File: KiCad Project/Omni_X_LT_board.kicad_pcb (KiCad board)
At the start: 2 copper layers, 64.8 x 25.5 mm, 32 parts, among them J1 Conn_01x02_Female, J2 Conn_01x02_Female, U1 TLV9001IDCK, U2 TLV9001IDCK, U3 ADS1110

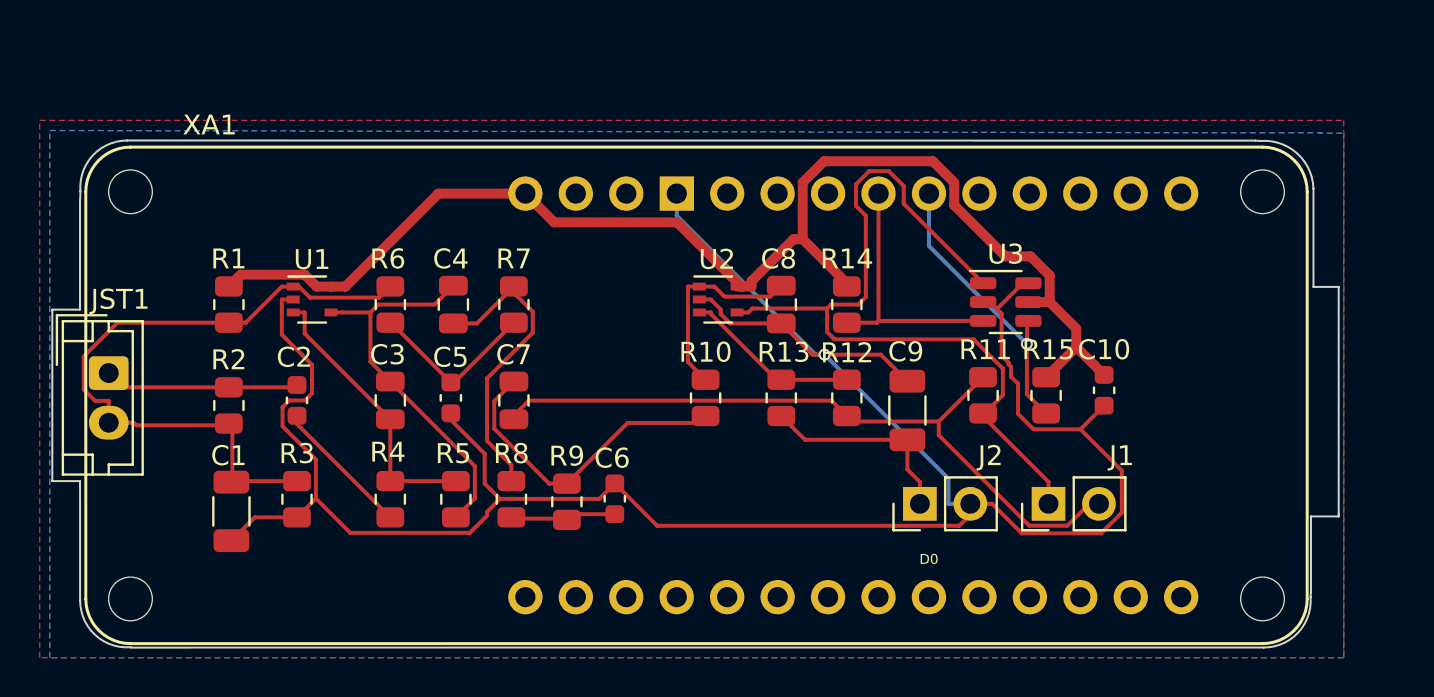
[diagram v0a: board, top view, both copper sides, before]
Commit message: update KiCad files
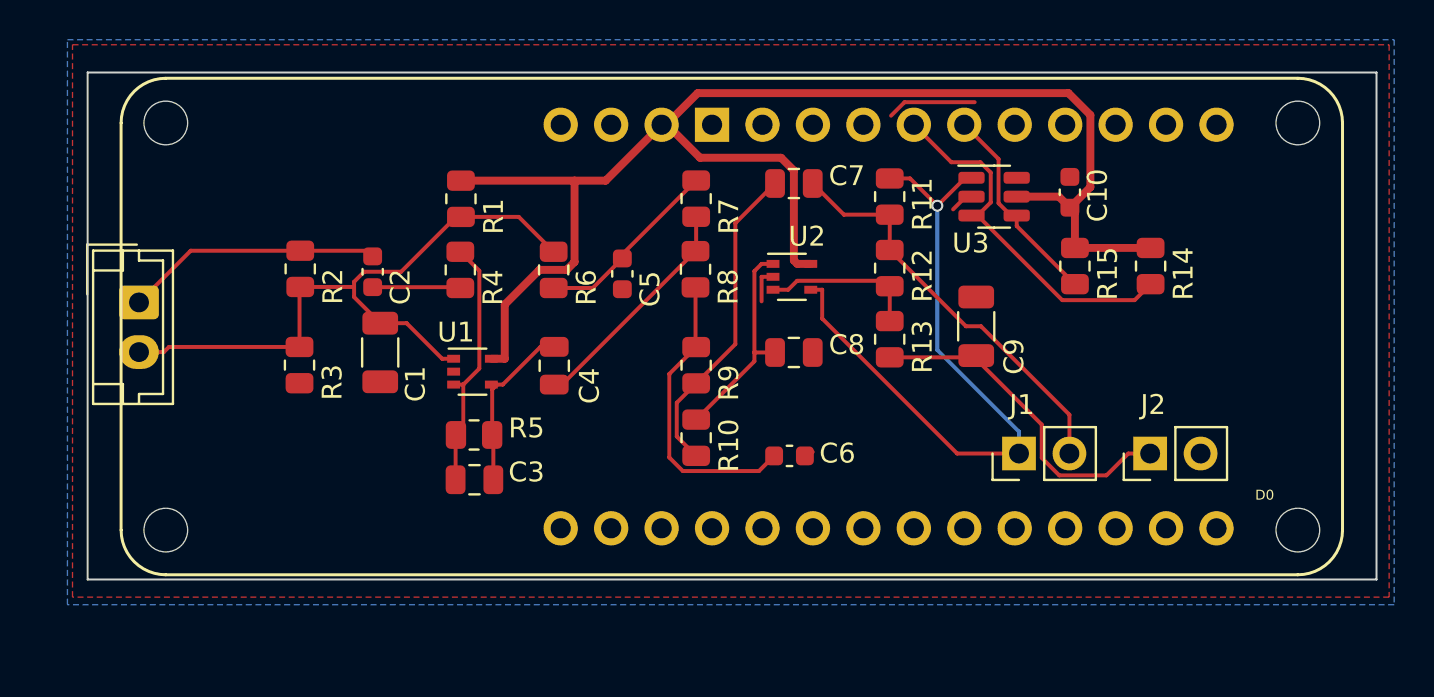
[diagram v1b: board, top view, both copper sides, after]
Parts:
- R2: value 1k -> 7.5k
- moved C7 17.8 mm to (151.5, 48.9), turned to 0 degrees
- moved R14 15.4 mm to (169.5, 53.1)
- moved R8 14.8 mm to (146.6, 53.2)
- moved R1 12.8 mm to (134.7, 49.7)
- moved R4 12.1 mm to (134.7, 53.2)
- moved J2 11.9 mm to (169.4, 62.5)
- moved R11 11.1 mm to (156.3, 49.6), turned to -90 degrees
- moved C1 11.0 mm to (130.7, 57.4)
- moved C5 10.7 mm to (142.9, 53.4)
- moved R7 10.6 mm to (146.6, 49.7), turned to 90 degrees
- moved C10 10.1 mm to (165.4, 49.3), turned to 90 degrees
- moved R9 9.47 mm to (146.6, 58.0), turned to 90 degrees
- moved C6 9.06 mm to (151.3, 62.6), turned to 0 degrees
- moved U1 8.85 mm to (135.3, 58.4)
- moved R6 8.41 mm to (139.4, 53.2)
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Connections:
- C10 pad 1: +5V -> 3V3
- R1 pad 1: +5V -> 3V3
- R14 pad 1: +5V -> 3V3
- R15 pad 1: +5V -> 3V3
- U1 pad 5: +5V -> 3V3
- U2 pad 5: +5V -> 3V3
- U3 pad 5: +5V -> 3V3
- XA1 pad 3V3: unconnected-(XA1-Pad3V3) -> 3V3
- XA1 pad 5V: +5V -> unconnected-(XA1-Pad5V)
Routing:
- net GND: track 122.7 -> 8.54 mm, vias 1 -> 0
- net 3V3: track 0.00 -> 72.6 mm
- net +5V: track 66.1 -> 0.00 mm
- net Net-(C7-Pad2): track 37.4 -> 20.7 mm
- net Net-(C3-Pad2): track 19.6 -> 8.87 mm
- net Net-(C6-Pad1): track 5.47 -> 15.0 mm
- net Net-(J1-Pad1): track 41.7 -> 34.2 mm, vias 0 -> 1
- net Net-(C9-Pad1): track 10.3 -> 17.1 mm
- net D12_SCL: track 13.3 -> 18.4 mm
- net D11_SDA: track 14.8 -> 10.5 mm, vias 1 -> 0
- net Net-(C4-Pad2): track 15.4 -> 11.6 mm
- net Net-(C2-Pad1): track 9.83 -> 13.0 mm
- net Net-(C2-Pad2): track 7.06 -> 4.43 mm
- net Net-(C3-Pad1): track 14.2 -> 12.9 mm
- net Net-(C1-Pad1): track 34.1 -> 33.1 mm
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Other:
- board size 64.8 x 25.5 mm -> 64.9 x 25.5 mm
